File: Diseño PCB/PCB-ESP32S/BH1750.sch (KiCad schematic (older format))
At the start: 7 parts, among them IC1 BH1750FVI-TR, J2 Screw_Terminal_01x05

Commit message: esp-32 actualizacion
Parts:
- R10, R7, R8, R9: footprint Resistor_SMD:R_0201_0603Metric -> Resistor_SMD:R_0805_2012Metric_Pad1.20x1.40mm_HandSolder
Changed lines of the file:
@@
 $Descr A4 11693 8268
 encoding utf-8
-Sheet 5 8
+Sheet 4 8
 Title ""
 Date ""
@@
 F 0 "R7" V 5143 2850 50  0000 C CNN
 F 1 "1k" V 5234 2850 50  0000 C CNN
-F 2 "Resistor_SMD:R_0201_0603Metric" V 5280 2850 50  0000 C CNN
+F 2 "Resistor_SMD:R_0805_2012Metric_Pad1.20x1.40mm_HandSolder" V 5280 2850 50  0000 C CNN
 F 3 "~" H 5350 2850 50  0001 C CNN
 	1    5350 2850
@@
 F 0 "R10" H 7420 3296 50  0000 L CNN
 F 1 "4.7k" H 7420 3205 50  0000 L CNN
-F 2 "Resistor_SMD:R_0201_0603Metric" V 7280 3250 50  0001 C CNN
+F 2 "Resistor_SMD:R_0805_2012Metric_Pad1.20x1.40mm_HandSolder" V 7280 3250 50  0001 C CNN
 F 3 "~" H 7350 3250 50  0001 C CNN
 	1    7350 3250
@@
 F 0 "R9" H 7070 3396 50  0000 L CNN
 F 1 "4.7k" H 7070 3305 50  0000 L CNN
-F 2 "Resistor_SMD:R_0201_0603Metric" V 6930 3350 50  0001 C CNN
+F 2 "Resistor_SMD:R_0805_2012Metric_Pad1.20x1.40mm_HandSolder" V 6930 3350 50  0001 C CNN
 F 3 "~" H 7000 3350 50  0001 C CNN
 	1    7000 3350
@@
 F 0 "R8" H 4670 3796 50  0000 L CNN
 F 1 "4.7k" H 4670 3705 50  0000 L CNN
-F 2 "Resistor_SMD:R_0201_0603Metric" V 4530 3750 50  0001 C CNN
+F 2 "Resistor_SMD:R_0805_2012Metric_Pad1.20x1.40mm_HandSolder" V 4530 3750 50  0001 C CNN
 F 3 "~" H 4600 3750 50  0001 C CNN
 	1    4600 3750

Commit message: .
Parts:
- IC1: symbol BH1750FVI-TR:BH1750FVI-TR -> PCB-ESP32S-rescue:BH1750FVI-TR-BH1750FVI-TR
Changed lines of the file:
@@
 $EndDescr
 $Comp
-L BH1750FVI-TR:BH1750FVI-TR IC1
+L PCB-ESP32S-rescue:BH1750FVI-TR-BH1750FVI-TR IC1
 U 1 1 61A84806
 P 5000 3500
+AR Path="/61A84806" Ref="IC1"  Part="1"
+AR Path="/61A843AA/61A84806" Ref="IC1"  Part="1"
 F 0 "IC1" H 5550 3765 50  0000 C CNN
 F 1 "BH1750FVI-TR" H 5550 3674 50  0000 C CNN

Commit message: Actualización footprints
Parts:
- IC1: symbol PCB-ESP32S-rescue:BH1750FVI-TR-BH1750FVI-TR -> PCB-ESP32S-rescue:BH1750FVI-TR-BH1750FVI-TR-PCB-ESP32S-rescue
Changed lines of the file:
@@
 $EndDescr
 $Comp
-L PCB-ESP32S-rescue:BH1750FVI-TR-BH1750FVI-TR IC1
+L PCB-ESP32S-rescue:BH1750FVI-TR-BH1750FVI-TR-PCB-ESP32S-rescue IC1
 U 1 1 61A84806
 P 5000 3500

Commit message: verificacion componentes
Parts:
- C1: footprint (none) -> Capacitor_SMD:C_0805_2012Metric_Pad1.18x1.45mm_HandSolder
- J2: footprint (none) -> Connector_JST:JST_GH_BM05B-GHS-TBT_1x05-1MP_P1.25mm_Vertical
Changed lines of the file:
@@
 F 0 "C1" H 6615 3796 50  0000 L CNN
 F 1 "0.1uF" H 6615 3705 50  0000 L CNN
-F 2 "" H 6538 3600 50  0001 C CNN
+F 2 "Capacitor_SMD:C_0805_2012Metric_Pad1.18x1.45mm_HandSolder" H 6538 3600 50  0001 C CNN
 F 3 "~" H 6500 3750 50  0001 C CNN
 	1    6500 3750
@@
 F 0 "J2" H 8330 3492 50  0000 L CNN
 F 1 "Screw_Terminal_01x05" H 8330 3401 50  0000 L CNN
-F 2 "" H 8250 3450 50  0001 C CNN
+F 2 "Connector_JST:JST_GH_BM05B-GHS-TBT_1x05-1MP_P1.25mm_Vertical" H 8250 3450 50  0001 C CNN
 F 3 "~" H 8250 3450 50  0001 C CNN
 	1    8250 3450

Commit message: LuzSens-actualización
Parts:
- removed J2: Screw_Terminal_01x05, Connector_JST:JST_GH_BM05B-GHS-TBT_1x05-1MP_P1.25mm_Vertical, symbol Connector:Screw_Terminal_01x05
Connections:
- wire segments 34 -> 27
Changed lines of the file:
@@
 Wire Wire Line
 	4600 3500 5000 3500
-$Comp
-L Device:C C1
-U 1 1 61A8B370
-P 6500 3750
-F 0 "C1" H 6615 3796 50  0000 L CNN
-F 1 "0.1uF" H 6615 3705 50  0000 L CNN
-F 2 "Capacitor_SMD:C_0805_2012Metric_Pad1.18x1.45mm_HandSolder" H 6538 3600 50  0001 C CNN
-F 3 "~" H 6500 3750 50  0001 C CNN
-	1    6500 3750
-	1    0    0    -1
-$EndComp
 Wire Wire Line
 	5000 3600 4850 3600
-Wire Wire Line
-	5500 2850 6500 2850
-Wire Wire Line
-	6500 2850 6500 3600
-Wire Wire Line
-	6500 3600 6100 3600
-Connection ~ 6500 3600
-$Comp
-L Connector:Screw_Terminal_01x05 J2
-U 1 1 61A8FB11
-P 8250 3450
-F 0 "J2" H 8330 3492 50  0000 L CNN
-F 1 "Screw_Terminal_01x05" H 8330 3401 50  0000 L CNN
-F 2 "Connector_JST:JST_GH_BM05B-GHS-TBT_1x05-1MP_P1.25mm_Vertical" H 8250 3450 50  0001 C CNN
-F 3 "~" H 8250 3450 50  0001 C CNN
-	1    8250 3450
-	1    0    0    -1
-$EndComp
-Text HLabel 7850 3250 0    50   Input ~ 0
-Vcc
-Text HLabel 7850 3350 0    50   Input ~ 0
-GND
-Text HLabel 7850 3450 0    50   Input ~ 0
-SCL
-Text HLabel 7850 3550 0    50   Input ~ 0
-SDA
-Text HLabel 7850 3650 0    50   Input ~ 0
-ADDR
-Wire Wire Line
-	8050 3350 7850 3350
-Wire Wire Line
-	8050 3450 7950 3450
-Wire Wire Line
-	8050 3550 7950 3550
 $Comp
 L Device:R R10
@@
 $EndComp
 Wire Wire Line
-	7950 3400 7950 3450
-Connection ~ 7950 3450
-Wire Wire Line
-	7950 3450 7850 3450
-Wire Wire Line
-	7950 3500 7950 3550
-Connection ~ 7950 3550
-Wire Wire Line
-	7950 3550 7850 3550
-Wire Wire Line
 	7000 3200 7000 3000
 Wire Wire Line
@@
 Wire Wire Line
 	7000 3000 7150 3000
-Wire Wire Line
-	7850 3650 8050 3650
 Text HLabel 7150 2900 1    50   Input ~ 0
 Vcc
@@
 Wire Wire Line
 	7150 3000 7350 3000
-Wire Wire Line
-	7850 3250 8050 3250
 Text HLabel 4400 2850 0    50   Input ~ 0
 Vcc
@@
 Wire Wire Line
 	4850 3600 4600 3600
-Text HLabel 6200 3500 2    50   Input ~ 0
-SCL
-Text HLabel 6200 3700 2    50   Input ~ 0
-SDA
 Wire Wire Line
 	6200 3500 6100 3500
-Wire Wire Line
-	6200 3700 6100 3700
 $Comp
 L Device:R R8
@@
 Connection ~ 4600 4250
 Wire Wire Line
-	5000 4250 6500 4250
+	6200 3700 6100 3700
+Text HLabel 7450 3750 2    50   Input ~ 0
+SCL
+Text HLabel 7450 3650 2    50   Input ~ 0
+SDA
+Connection ~ 5000 4250
 Wire Wire Line
 	6500 4250 6500 3900
-Connection ~ 5000 4250
 Wire Wire Line
-	7350 3400 7950 3400
+	5000 4250 6500 4250
+Text HLabel 6200 3700 2    50   Input ~ 0
+SDA
+Text HLabel 6200 3500 2    50   Input ~ 0
+SCL
+Connection ~ 6500 3600
 Wire Wire Line
-	7000 3500 7950 3500
+	6500 3600 6100 3600
+Wire Wire Line
+	6500 2850 6500 3600
+Wire Wire Line
+	5500 2850 6500 2850
+$Comp
+L Device:C C1
+U 1 1 61A8B370
+P 6500 3750
+F 0 "C1" H 6615 3796 50  0000 L CNN
+F 1 "0.1uF" H 6615 3705 50  0000 L CNN
+F 2 "Capacitor_SMD:C_0805_2012Metric_Pad1.18x1.45mm_HandSolder" H 6538 3600 50  0001 C CNN
+F 3 "~" H 6500 3750 50  0001 C CNN
+	1    6500 3750
+	1    0    0    -1
+$EndComp
+Wire Wire Line
+	7350 3400 7350 3650
+Wire Wire Line
+	7350 3650 7450 3650
+Wire Wire Line
+	7450 3750 7000 3750
+Wire Wire Line
+	7000 3750 7000 3500
 $EndSCHEMATC

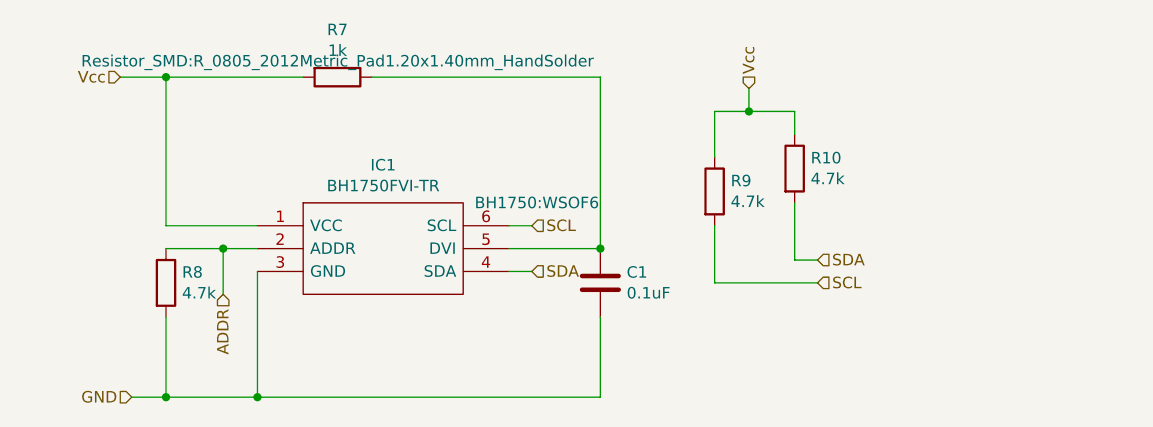
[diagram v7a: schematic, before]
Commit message: PCBs ok
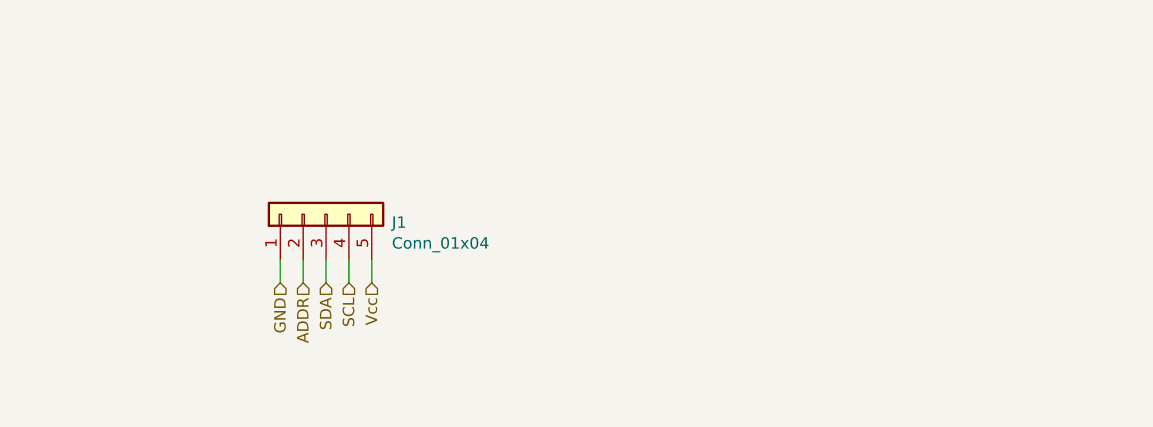
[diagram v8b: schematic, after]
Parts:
- removed C1: 0.1uF, Capacitor_SMD:C_0805_2012Metric_Pad1.18x1.45mm_HandSolder, symbol Device:C
- removed IC1: BH1750FVI-TR, BH1750:WSOF6, symbol PCB-ESP32S-rescue:BH1750FVI-TR-BH1750FVI-TR-PCB-ESP32S-rescue
- removed R10, R8, R9: 4.7k, Resistor_SMD:R_0805_2012Metric_Pad1.20x1.40mm_HandSolder, symbol Device:R
- removed R7: 1k, Resistor_SMD:R_0805_2012Metric_Pad1.20x1.40mm_HandSolder, symbol Device:R
- added J1: Conn_01x04, Connector_JST:JST_EH_B5B-EH-A_1x05_P2.50mm_Vertical, symbol Connector_Generic:Conn_01x05
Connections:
- net ADDR: now also J1.2 (Pin_2)
- net GND: now also J1.1 (Pin_1)
- net SCL: now also J1.4 (Pin_4)
- net SDA: now also J1.3 (Pin_3)
- net Vcc: now also J1.5 (Pin_5)
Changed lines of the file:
@@
 $EndDescr
 $Comp
-L PCB-ESP32S-rescue:BH1750FVI-TR-BH1750FVI-TR-PCB-ESP32S-rescue IC1
-U 1 1 61A84806
-P 5000 3500
-AR Path="/61A84806" Ref="IC1"  Part="1"
-AR Path="/61A843AA/61A84806" Ref="IC1"  Part="1"
-F 0 "IC1" H 5550 3765 50  0000 C CNN
-F 1 "BH1750FVI-TR" H 5550 3674 50  0000 C CNN
-F 2 "BH1750:WSOF6" H 5950 3600 50  0000 L CNN
-F 3 "https://componentsearchengine.com/Datasheets/2/BH1750FVI-TR.pdf" H 5950 3500 50  0001 L CNN
-F 4 "Ambient Light Sensor,16bit,I2C,WSOF6I ROHM BH1750FVI-TR Ambient Light Sensor Unit Surface Mount" H 5950 3400 50  0001 L CNN "Description"
-F 5 "" H 5950 3300 50  0001 L CNN "Height"
-F 6 "ROHM Semiconductor" H 5950 3200 50  0001 L CNN "Manufacturer_Name"
-F 7 "BH1750FVI-TR" H 5950 3100 50  0001 L CNN "Manufacturer_Part_Number"
-F 8 "755-BH1750FVI-TR" H 5950 3000 50  0001 L CNN "Mouser Part Number"
-F 9 "https://www.mouser.co.uk/ProductDetail/ROHM-Semiconductor/BH1750FVI-TR?qs=phc6PQ%252BTPUNy88lRCs6mVA%3D%3D" H 5950 2900 50  0001 L CNN "Mouser Price/Stock"
-F 10 "BH1750FVI-TR" H 5950 2800 50  0001 L CNN "Arrow Part Number"
-F 11 "https://www.arrow.com/en/products/bh1750fvi-tr/rohm-semiconductor" H 5950 2700 50  0001 L CNN "Arrow Price/Stock"
-	1    5000 3500
-	1    0    0    -1
+L Connector_Generic:Conn_01x05 J1
+U 1 1 61E257B3
+P 5300 3450
+AR Path="/61A843AA/61E257B3" Ref="J1"  Part="1"
+AR Path="/61A90AD5/61E257B3" Ref="BH1750"  Part="1"
+F 0 "J1" V 5264 3162 50  0000 R CNN
+F 1 "Conn_01x04" V 5173 3162 50  0000 R CNN
+F 2 "Connector_JST:JST_EH_B5B-EH-A_1x05_P2.50mm_Vertical" H 5300 3450 50  0001 C CNN
+F 3 "~" H 5300 3450 50  0001 C CNN
+	1    5300 3450
+	0    -1   -1   0
 $EndComp
-$Comp
-L Device:R R7
-U 1 1 61A8A6CD
-P 5350 2850
-F 0 "R7" V 5143 2850 50  0000 C CNN
-F 1 "1k" V 5234 2850 50  0000 C CNN
-F 2 "Resistor_SMD:R_0805_2012Metric_Pad1.20x1.40mm_HandSolder" V 5280 2850 50  0000 C CNN
-F 3 "~" H 5350 2850 50  0001 C CNN
-	1    5350 2850
-	0    1    1    0
-$EndComp
-Wire Wire Line
-	5200 2850 4600 2850
-Wire Wire Line
-	4600 2850 4600 3500
-Wire Wire Line
-	4600 3500 5000 3500
-Wire Wire Line
-	5000 3600 4850 3600
-$Comp
-L Device:R R10
-U 1 1 61A9346F
-P 7350 3250
-F 0 "R10" H 7420 3296 50  0000 L CNN
-F 1 "4.7k" H 7420 3205 50  0000 L CNN
-F 2 "Resistor_SMD:R_0805_2012Metric_Pad1.20x1.40mm_HandSolder" V 7280 3250 50  0001 C CNN
-F 3 "~" H 7350 3250 50  0001 C CNN
-	1    7350 3250
-	1    0    0    -1
-$EndComp
-$Comp
-L Device:R R9
-U 1 1 61A93EDA
-P 7000 3350
-F 0 "R9" H 7070 3396 50  0000 L CNN
-F 1 "4.7k" H 7070 3305 50  0000 L CNN
-F 2 "Resistor_SMD:R_0805_2012Metric_Pad1.20x1.40mm_HandSolder" V 6930 3350 50  0001 C CNN
-F 3 "~" H 7000 3350 50  0001 C CNN
-	1    7000 3350
-	1    0    0    -1
-$EndComp
-Wire Wire Line
-	7000 3200 7000 3000
-Wire Wire Line
-	7350 3000 7350 3100
-Wire Wire Line
-	7000 3000 7150 3000
-Text HLabel 7150 2900 1    50   Input ~ 0
+Text HLabel 5100 3750 3    50   Input ~ 0
+GND
+Text HLabel 5200 3750 3    50   Input ~ 0
+ADDR
+Text HLabel 5300 3750 3    50   Input ~ 0
+SDA
+Text HLabel 5400 3750 3    50   Input ~ 0
+SCL
+Text HLabel 5500 3750 3    50   Input ~ 0
 Vcc
 Wire Wire Line
-	7150 2900 7150 3000
-Connection ~ 7150 3000
+	5500 3650 5500 3750
 Wire Wire Line
-	7150 3000 7350 3000
-Text HLabel 4400 2850 0    50   Input ~ 0
-Vcc
+	5400 3650 5400 3750
 Wire Wire Line
-	4400 2850 4600 2850
-Connection ~ 4600 2850
-Text HLabel 4850 3800 3    50   Input ~ 0
-ADDR
+	5300 3650 5300 3750
 Wire Wire Line
-	4850 3800 4850 3600
-Connection ~ 4850 3600
+	5200 3650 5200 3750
 Wire Wire Line
-	4850 3600 4600 3600
-Wire Wire Line
-	6200 3500 6100 3500
-$Comp
-L Device:R R8
-U 1 1 61A8BE3F
-P 4600 3750
-F 0 "R8" H 4670 3796 50  0000 L CNN
-F 1 "4.7k" H 4670 3705 50  0000 L CNN
-F 2 "Resistor_SMD:R_0805_2012Metric_Pad1.20x1.40mm_HandSolder" V 4530 3750 50  0001 C CNN
-F 3 "~" H 4600 3750 50  0001 C CNN
-	1    4600 3750
-	1    0    0    -1
-$EndComp
-Text HLabel 4450 4250 0    50   Input ~ 0
-GND
-Wire Wire Line
-	4600 3900 4600 4250
-Wire Wire Line
-	4600 4250 4450 4250
-Wire Wire Line
-	4600 4250 5000 4250
-Wire Wire Line
-	5000 4250 5000 3700
-Connection ~ 4600 4250
-Wire Wire Line
-	6200 3700 6100 3700
-Text HLabel 7450 3750 2    50   Input ~ 0
-SCL
-Text HLabel 7450 3650 2    50   Input ~ 0
-SDA
-Connection ~ 5000 4250
-Wire Wire Line
-	6500 4250 6500 3900
-Wire Wire Line
-	5000 4250 6500 4250
-Text HLabel 6200 3700 2    50   Input ~ 0
-SDA
-Text HLabel 6200 3500 2    50   Input ~ 0
-SCL
-Connection ~ 6500 3600
-Wire Wire Line
-	6500 3600 6100 3600
-Wire Wire Line
-	6500 2850 6500 3600
-Wire Wire Line
-	5500 2850 6500 2850
-$Comp
-L Device:C C1
-U 1 1 61A8B370
-P 6500 3750
-F 0 "C1" H 6615 3796 50  0000 L CNN
-F 1 "0.1uF" H 6615 3705 50  0000 L CNN
-F 2 "Capacitor_SMD:C_0805_2012Metric_Pad1.18x1.45mm_HandSolder" H 6538 3600 50  0001 C CNN
-F 3 "~" H 6500 3750 50  0001 C CNN
-	1    6500 3750
-	1    0    0    -1
-$EndComp
-Wire Wire Line
-	7350 3400 7350 3650
-Wire Wire Line
-	7350 3650 7450 3650
-Wire Wire Line
-	7450 3750 7000 3750
-Wire Wire Line
-	7000 3750 7000 3500
+	5100 3650 5100 3750
 $EndSCHEMATC
